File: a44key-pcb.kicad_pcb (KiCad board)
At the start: 2 copper layers, 125.4 x 104 mm, 61 parts, among them J1 AudioJack3, SW1 SW_Push, U1 ATmega32U4-AU, Y1 16MHz

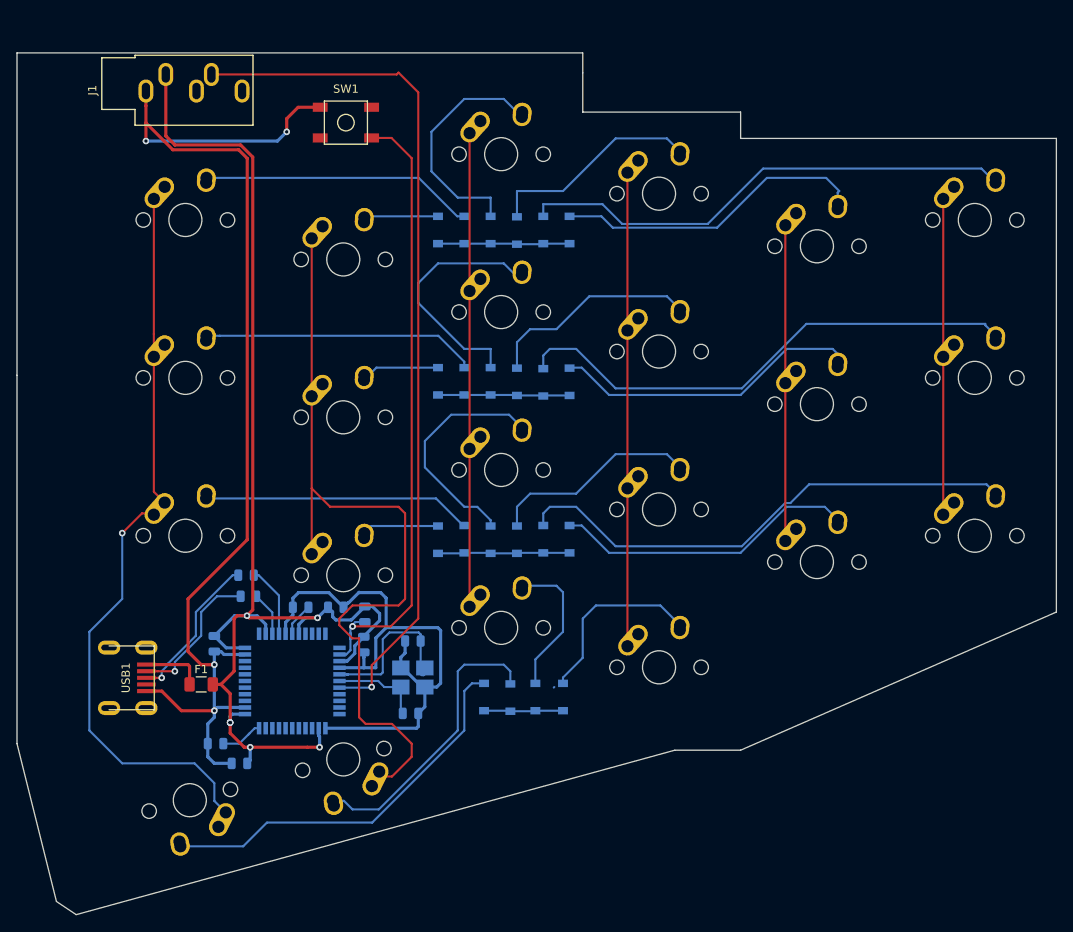
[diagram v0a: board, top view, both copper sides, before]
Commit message: Rewired
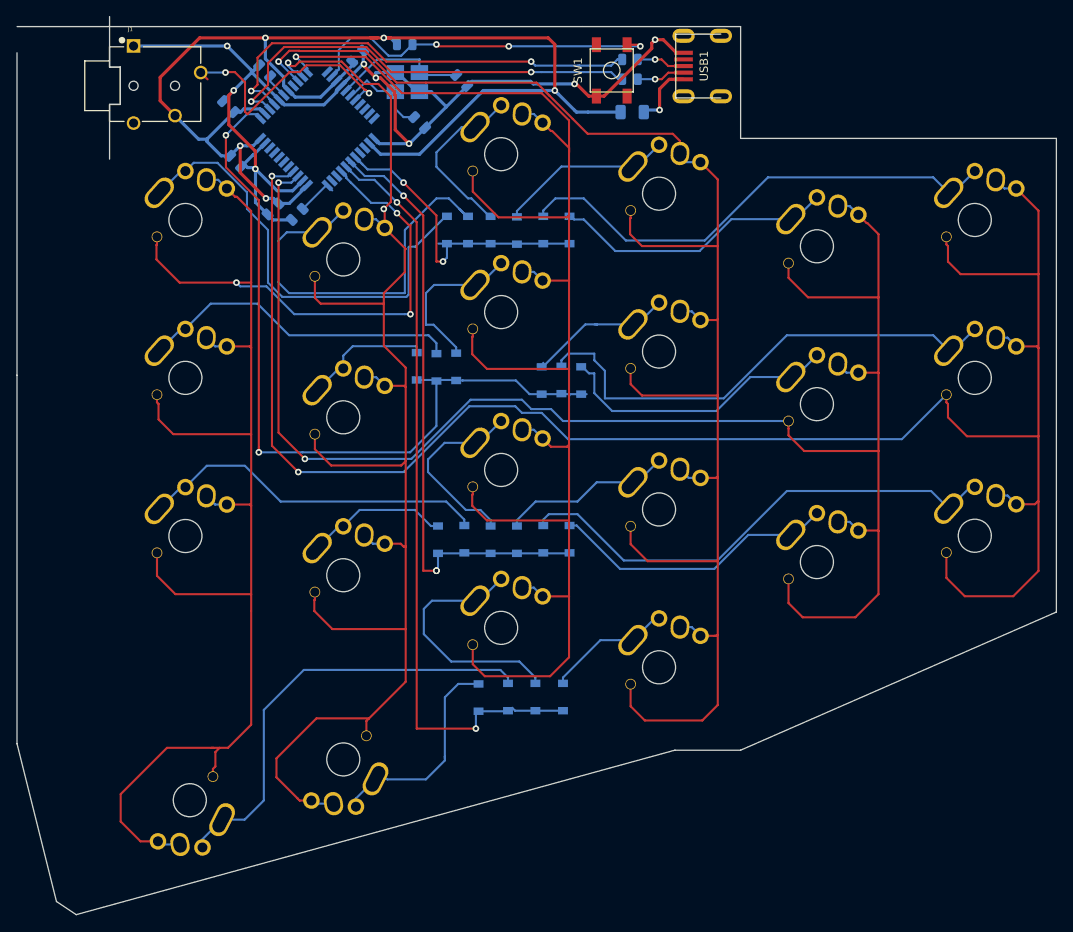
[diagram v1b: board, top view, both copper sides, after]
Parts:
- F1: moved to B.Cu
- J1: footprint Connector_Audio:Jack_3.5mm_CUI_SJ1-3535NG_Horizontal -> SJ-43514:CUI_SJ-43514
- MX1, MX10, MX11, MX12, MX13, MX14, MX15, MX16, MX17, MX18, MX19, MX2, MX20, MX21, MX22, MX3, MX4, MX5, MX6, MX7, MX8, MX9: footprint MX_Alps_Hybrid:MX-1U-NoLED -> MX_Alps_Hybrid:MX-Alps-Choc-X-1U-NoLED
- moved USB1 104.4 mm to (159.5, 51.6), turned to 180 degrees
- moved F1 86.4 mm to (148.8, 57.1)
- moved R2 77.6 mm to (148.6, 50.8), turned to 0 degrees
- moved R1 77.5 mm to (148.6, 53.2), turned to 0 degrees
- moved C5 72.6 mm to (101.0, 63.1), turned to 315 degrees
- moved Y1 71.8 mm to (121.7, 53.5)
- moved C2 71.3 mm to (123.2, 58.4), turned to 315 degrees
- moved R3 68.9 mm to (121.4, 49.0), turned to 0 degrees
- moved C3 67.9 mm to (128.3, 53.3), turned to 315 degrees
- moved C7 66.9 mm to (100.1, 56.5), turned to 135 degrees
- moved U1 66.7 mm to (110.8, 59.1), turned to 315 degrees
- moved C4 66.6 mm to (115.7, 50.4), turned to 45 degrees
- moved C6 64.9 mm to (104.5, 52.2), turned to 135 degrees
- moved R4 64.6 mm to (108.4, 69.5), turned to 45 degrees
- moved C1 52.9 mm to (105.5, 68.8), turned to 225 degrees
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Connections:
- U1 pad 1: Net-(U1-Pad1) -> ROW1
- U1 pad 10: Net-(U1-Pad10) -> COL4
- U1 pad 11: Net-(U1-Pad11) -> COL3
- U1 pad 27: Net-(U1-Pad27) -> ROW0
- U1 pad 28: Net-(U1-Pad28) -> ROW2
- U1 pad 29: Net-(U1-Pad29) -> ROW3
- U1 pad 30: Net-(U1-Pad30) -> COL5
- U1 pad 36: Net-(U1-Pad36) -> COL1
- U1 pad 37: Net-(U1-Pad37) -> COL0
- U1 pad 9: Net-(U1-Pad9) -> COL2
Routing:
- net COL0: track 38.7 -> 232.4 mm, vias 0 -> 2
- net COL1: track 38.1 -> 202.8 mm, vias 0 -> 2
- net COL2: track 57.2 -> 198.3 mm, vias 0 -> 1
- net COL3: track 57.2 -> 191.2 mm, vias 0 -> 1
- net COL5: track 90.7 -> 205.5 mm, vias 1 -> 3
- net ROW3: track 9.58 -> 93.2 mm, vias 0 -> 2
- net ROW1: track 16.0 -> 94.9 mm, vias 0 -> 2
- net COL4: track 100.1 -> 176.8 mm, vias 0 -> 2
- net SCL: track 104.0 -> 31.7 mm, vias 1 -> 2
- net GND: track 215.1 -> 145.9 mm, vias 4 -> 8
- net ROW2: track 16.0 -> 74.5 mm, vias 0 -> 3
- net Net-(R1-Pad1): track 5.33 -> 53.5 mm, vias 0 -> 2
- net Net-(R2-Pad1): track 8.66 -> 54.3 mm, vias 0 -> 2
- net Net-(D5-Pad2): track 8.94 -> 49.1 mm
- net Net-(R3-Pad2): track 75.2 -> 44.8 mm, vias 1 -> 3
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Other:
- board size 125.4 x 104 mm -> 125.4 x 107.2 mm
